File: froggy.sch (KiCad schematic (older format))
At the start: 14 parts, among them J1 USB_C_Receptacle_USB2.0, J2 Micro_SD_Card, U1 FT232RL, U2 LEAPSTER-CART

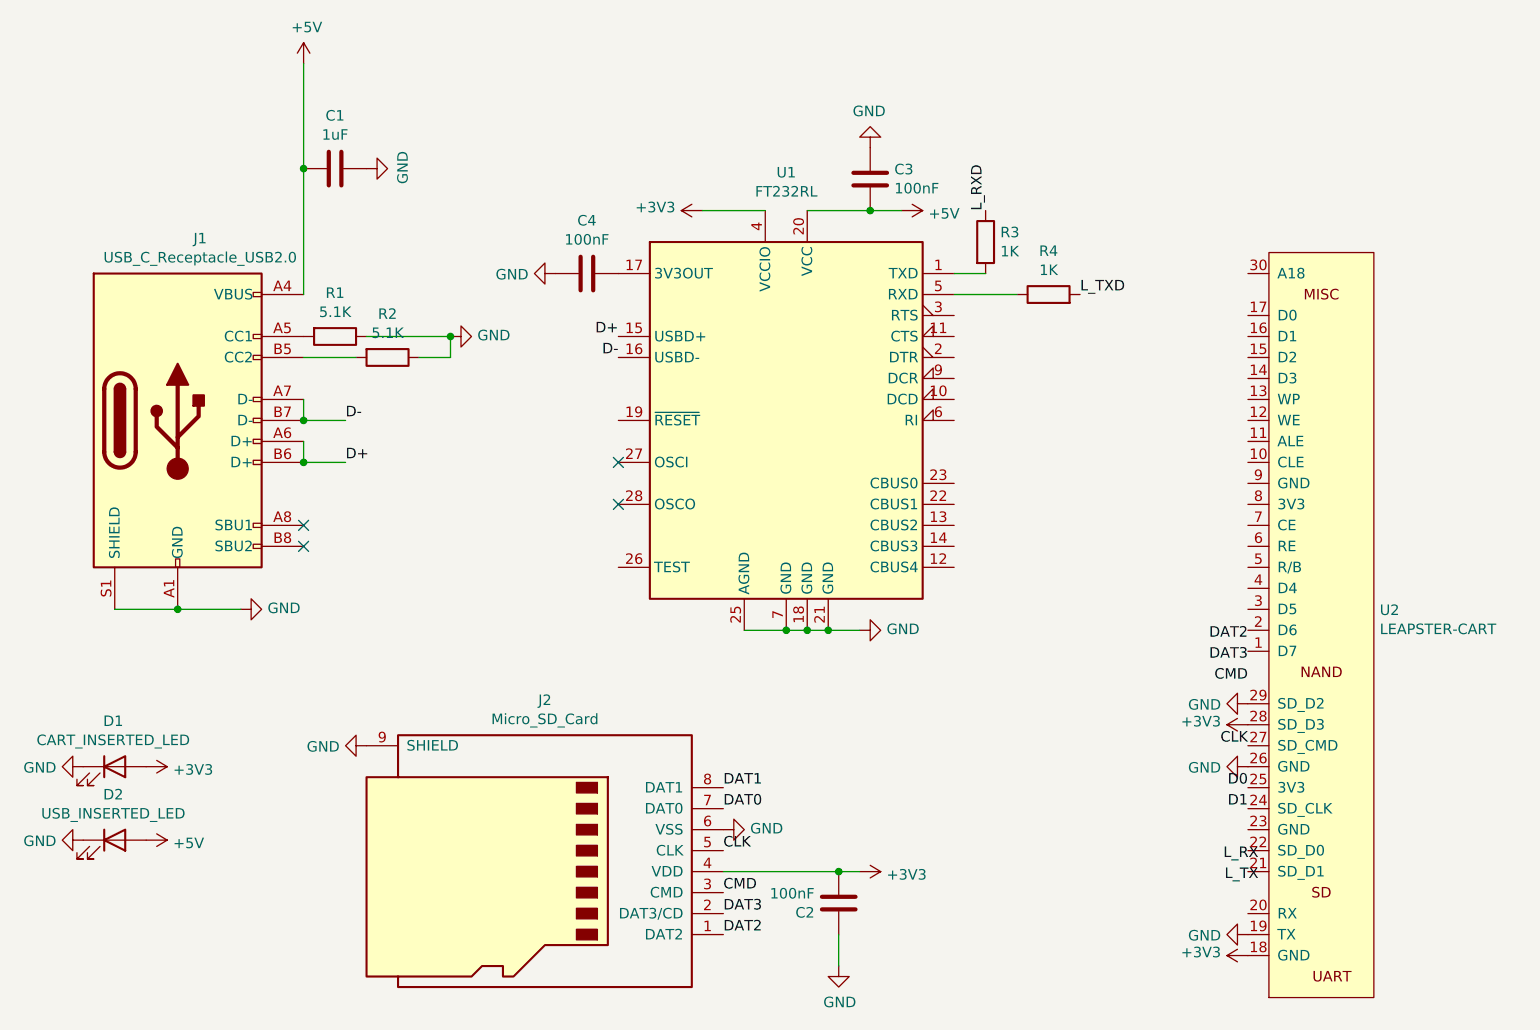
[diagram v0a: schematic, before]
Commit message: [upload] beautification
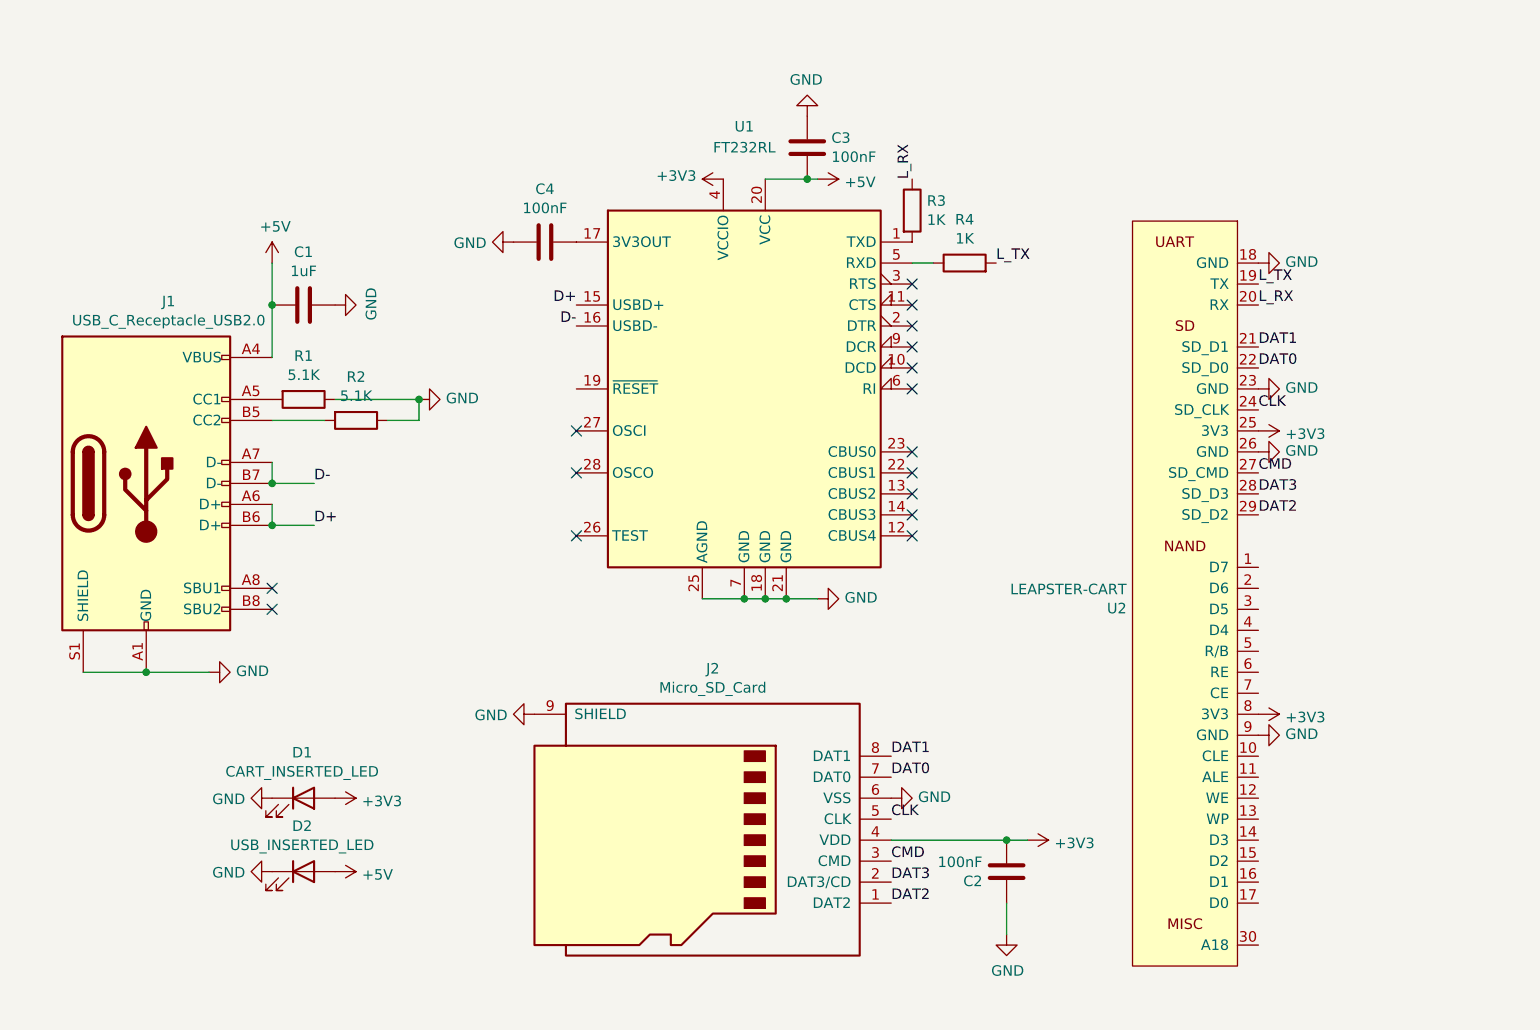
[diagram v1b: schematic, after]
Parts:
- C1, C2, C3, C4: footprint (none) -> Capacitor_SMD:C_0603_1608Metric
- D1, D2: footprint (none) -> Diode_SMD:D_0603_1608Metric
- J1: footprint (none) -> Connector_USB:USB_C_Receptacle_GCT_USB4085
- J2: footprint (none) -> SamacSys_Parts:5040771891
- R1, R2, R3, R4: footprint (none) -> Resistor_SMD:R_0603_1608Metric
- U2: footprint (none) -> Leapster:LEAPSTER_CART
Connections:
- net D0 is gone; now on net +3V3: U2.25 (3V3)
- net D1 is gone; now on net CLK: U2.24 (SD_CLK)
- net L_RXD is gone; now on net L_RX: R3.1
- net L_TXD is gone; now on net L_TX: R4.2
- net +3V3: now also U2.8 (3V3); no longer U2.18 (GND), U2.28 (SD_D3)
- net CLK: no longer U2.27 (SD_CMD)
- net CMD: now also U2.27 (SD_CMD)
- net DAT0: now also U2.22 (SD_D0)
- net DAT1: now also U2.21 (SD_D1)
- net DAT2: now also U2.29 (SD_D2)
- net DAT3: now also U2.28 (SD_D3)
- net GND: now also U2.18 (GND), U2.23 (GND), U2.9 (GND); no longer U2.19 (TX), U2.29 (SD_D2)
- net L_RX: now also U2.20 (RX)
- net L_TX: now also U2.19 (TX)
- no-connect marks 4 -> 16
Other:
- moved on the sheet: C1, C2, C3, C4, D1, D2, J1, J2, R1, R2, R3, R4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
